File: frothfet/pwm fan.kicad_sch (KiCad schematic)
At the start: 6 parts, among them M1 Fan_Tacho, Q9 AO3400A

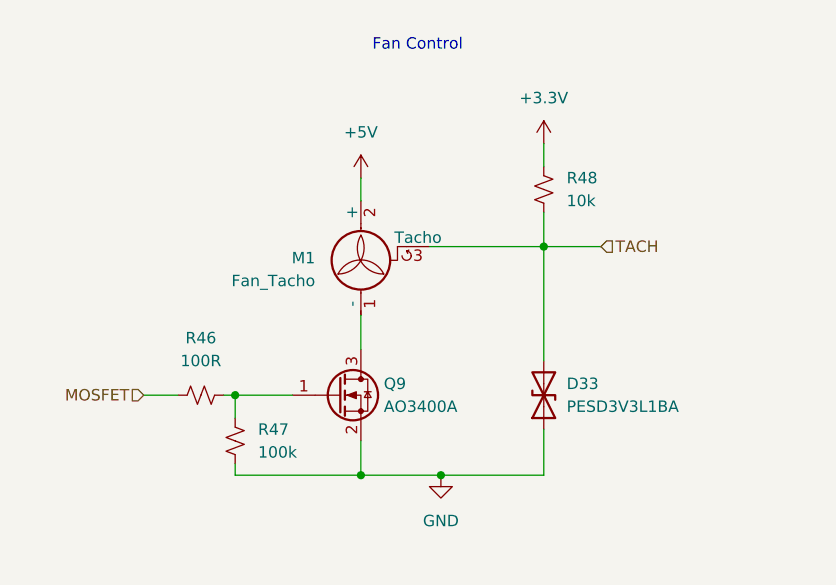
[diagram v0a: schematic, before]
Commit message: finished vias, added a bunch of test points
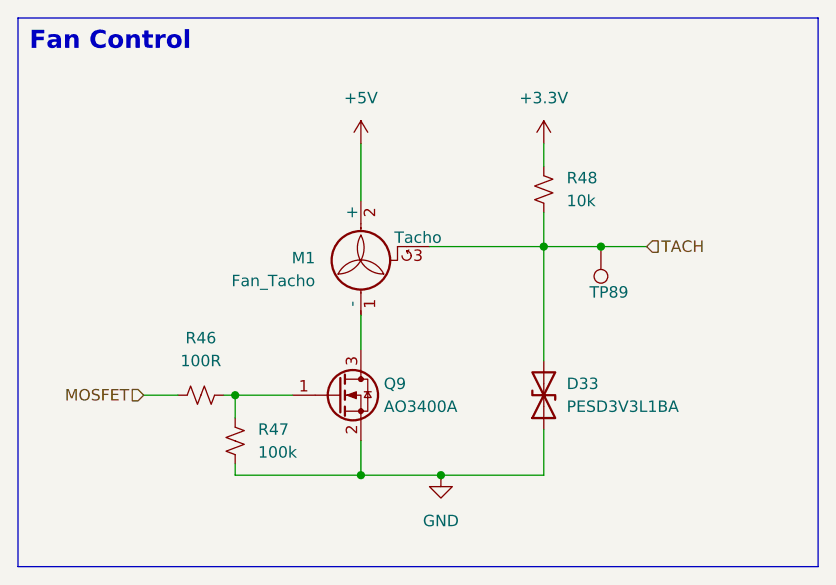
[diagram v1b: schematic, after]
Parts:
- added TP89: TestPoint, TestPoint:TestPoint_Pad_D1.5mm, symbol Connector:TestPoint
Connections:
- net TACH: now also TP89.1
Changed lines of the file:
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@@
 		(company "https://github.com/hoeken/frothfet")
+	)
+	(rectangle
+		(start 95.25 54.61)
+		(end 184.15 115.57)
+		(stroke
+			(width 0)
+			(type default)
+		)
+		(fill
+			(type none)
+		)
 	)
 	(text "Fan Control"
 		(exclude_from_sim no)
-		(at 134.62 58.42 0)
+		(at 96.52 58.42 0)
 		(effects
 			(font
-				(size 1.27 1.27)
+				(size 2 2)
+				(thickness 0.4)
+				(bold yes)
 			)
 			(justify left bottom)
@@
 		(color 0 0 0 0)
 	)
+	(junction
+		(at 160.02 80.01)
+		(diameter 0)
+		(color 0 0 0 0)
+	)
 	(wire
 		(pts
@@
 	(wire
 		(pts
+			(xy 160.02 80.01) (xy 165.1 80.01)
+		)
+		(stroke
+			(width 0)
+			(type default)
+		)
+	)
+	(wire
+		(pts
 			(xy 118.11 96.52) (xy 119.38 96.52)
 		)
@@
 	(wire
 		(pts
-			(xy 133.35 72.39) (xy 133.35 74.93)
+			(xy 133.35 68.58) (xy 133.35 74.93)
 		)
 		(stroke
@@
 	(hierarchical_label "TACH"
 		(shape input)
-		(at 160.02 80.01 0)
+		(at 165.1 80.01 0)
 		(effects
 			(font
@@
 				(path "/c83c6236-96e9-46ad-9d7a-9e2efa4a7966/ad82ad0c-2ba8-4934-bb2a-ed6e11658eb2"
 					(reference "D33")
+					(unit 1)
+				)
+			)
+		)
+	)
+	(symbol
+		(lib_id "Connector:TestPoint")
+		(at 160.02 80.01 0)
+		(mirror x)
+		(unit 1)
+		(exclude_from_sim no)
+		(in_bom yes)
+		(on_board yes)
+		(dnp no)
+		(property "Reference" "TP89"
+			(at 158.75 85.09 0)
+			(effects
+				(font
+					(size 1.27 1.27)
+				)
+				(justify left)
+			)
+		)
+		(property "Value" "TestPoint"
+			(at 162.56 82.0421 0)
+			(effects
+				(font
+					(size 1.27 1.27)
+				)
+				(justify left)
+				(hide yes)
+			)
+		)
+		(property "Footprint" "TestPoint:TestPoint_Pad_D1.5mm"
+			(at 165.1 80.01 0)
+			(effects
+				(font
+					(size 1.27 1.27)
+				)
+				(hide yes)
+			)
+		)
+		(property "Datasheet" "~"
+			(at 165.1 80.01 0)
+			(effects
+				(font
+					(size 1.27 1.27)
+				)
+				(hide yes)
+			)
+		)
+		(property "Description" "test point"
+			(at 160.02 80.01 0)
+			(effects
+				(font
+					(size 1.27 1.27)
+				)
+				(hide yes)
+			)
+		)
+		(pin "1"
+		)
+		(instances
+			(project "frothfet"
+				(path "/c83c6236-96e9-46ad-9d7a-9e2efa4a7966/02f6e629-b0e2-41e8-b2e4-f0e125a92a71"
+					(reference "TP90")
+					(unit 1)
+				)
+				(path "/c83c6236-96e9-46ad-9d7a-9e2efa4a7966/ad82ad0c-2ba8-4934-bb2a-ed6e11658eb2"
+					(reference "TP89")
 					(unit 1)
 				)
@@
 	(symbol
 		(lib_id "power:+5V")
-		(at 133.35 72.39 0)
+		(at 133.35 68.58 0)
 		(unit 1)
 		(exclude_from_sim no)
@@
 		(fields_autoplaced yes)
 		(property "Reference" "#PWR0125"
-			(at 133.35 76.2 0)
+			(at 133.35 72.39 0)
 			(effects
 				(font
@@
 		)
 		(property "Value" "+5V"
-			(at 133.35 67.31 0)
+			(at 133.35 63.5 0)
 			(effects
 				(font
@@
 		)
 		(property "Footprint" ""
-			(at 133.35 72.39 0)
+			(at 133.35 68.58 0)
 			(effects
 				(font
@@
 		)
 		(property "Datasheet" ""
-			(at 133.35 72.39 0)
+			(at 133.35 68.58 0)
 			(effects
 				(font
@@
 		)
 		(property "Description" "Power symbol creates a global label with name \"+5V\""
-			(at 133.35 72.39 0)
-			(effects
-				(font
+			(at 133.35 68.58 0)
+			(effects
+				(font
